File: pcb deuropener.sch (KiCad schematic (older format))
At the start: 30 parts, among them J1 Conn_01x02, J10 Conn_01x03, J11 Barrel_Jack_Switch, J12 Conn_01x08, J13 Conn_01x02, J14 Conn_01x02, J2 Conn_01x02, J3 Conn_01x02, J4 Conn_01x02, J8 Conn_01x02, P8 BeagleBone_Black_Header, P9 BeagleBone_Black_Header, Q1 STU60N3LH5, U1 TSR_1-2450

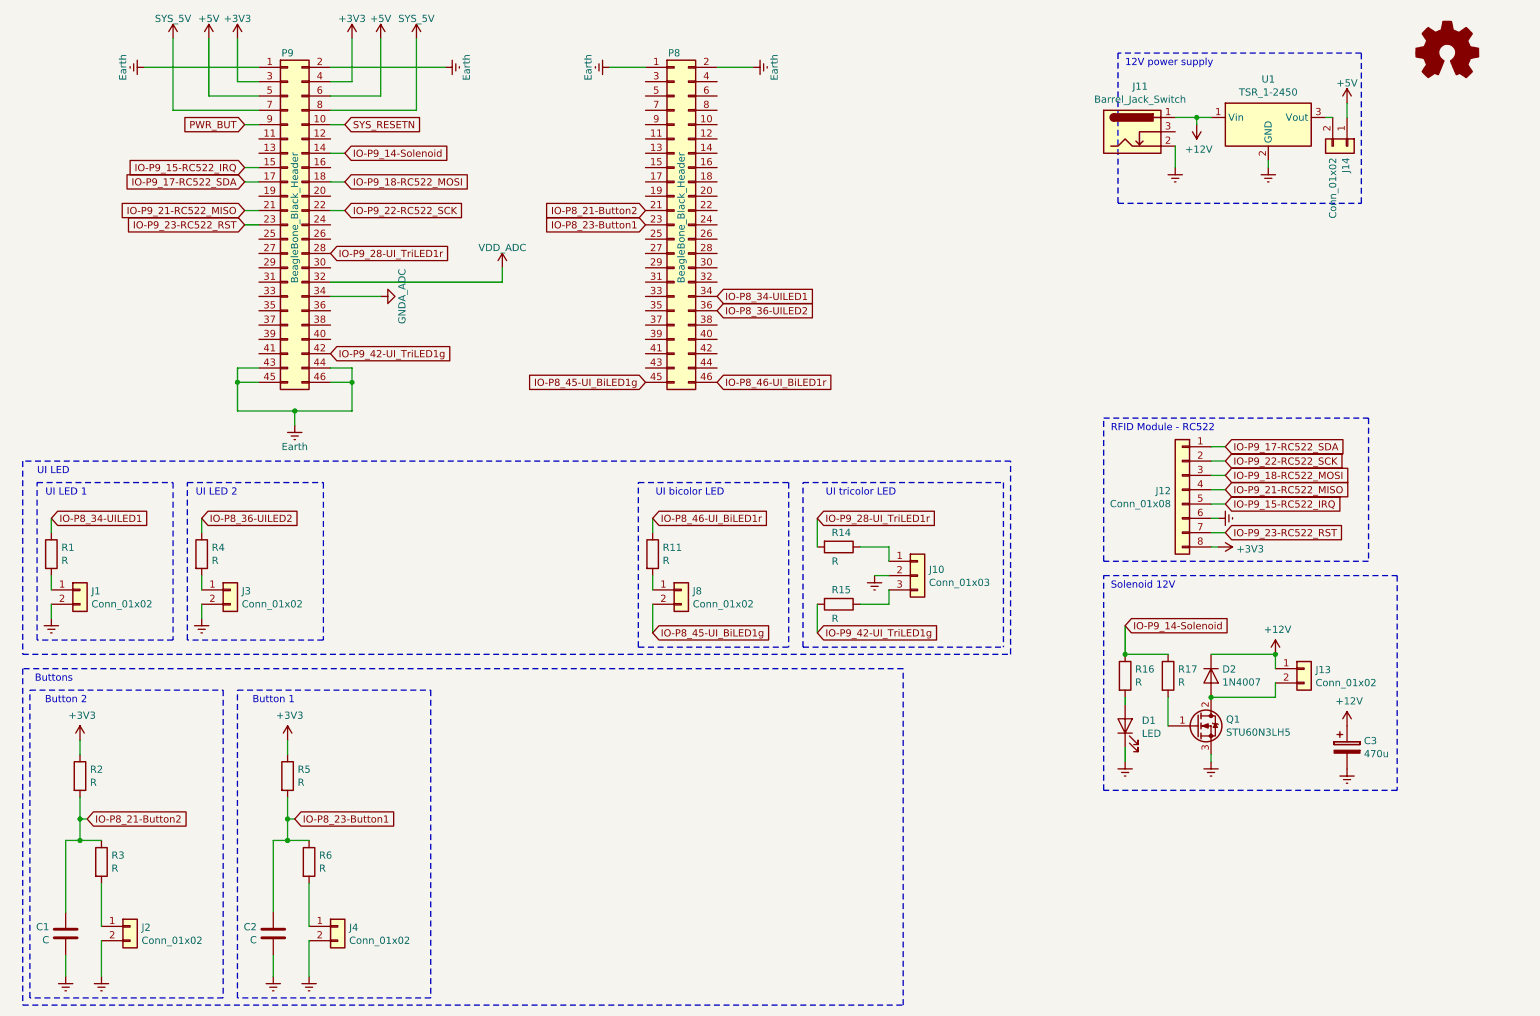
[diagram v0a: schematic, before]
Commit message: A lot of changes to rev 0.02
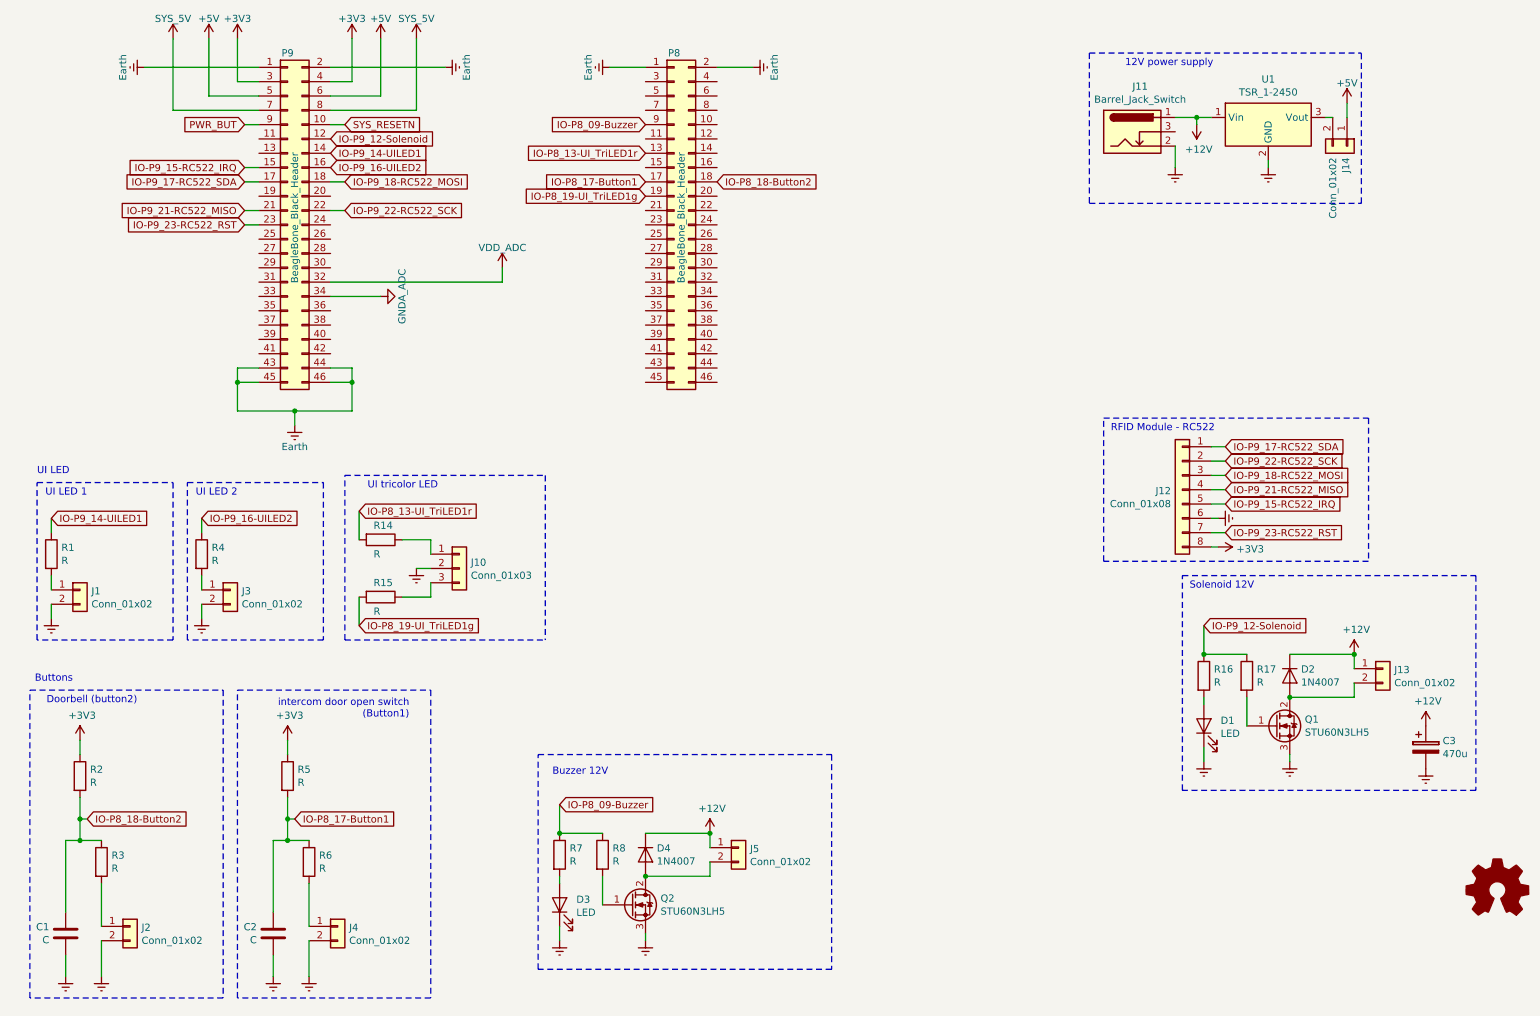
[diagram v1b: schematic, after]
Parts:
- removed J8: Conn_01x02, Connector_PinHeader_2.54mm:PinHeader_1x02_P2.54mm_Vertical, symbol Connector_Generic:Conn_01x02
- removed R11: R, Resistor_THT:R_Axial_DIN0207_L6.3mm_D2.5mm_P10.16mm_Horizontal, symbol Device:R
- added D3: LED, LED_THT:LED_D5.0mm, symbol Device:LED
- added D4: 1N4007, Diode_THT:D_DO-41_SOD81_P10.16mm_Horizontal, symbol Diode:1N4007
- added J5: Conn_01x02, Connector_PinHeader_2.54mm:PinHeader_1x02_P2.54mm_Vertical, symbol Connector_Generic:Conn_01x02
- added Q2: STU60N3LH5, Package_TO_SOT_THT:SIPAK_Vertical, symbol Device:Q_NMOS_GDS
- added R7, R8: R, Resistor_THT:R_Axial_DIN0207_L6.3mm_D2.5mm_P10.16mm_Horizontal, symbol Device:R
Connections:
- net +12V: now also D4.1 (K), J5.1 (Pin_1)
- net Earth: now also D3.1 (K), Q2.3 (S)
- net IO-P9_12-Solenoid: now reaches P9.12 (Pin_12)
- net IO-P9_12-Solenoid: now also R16.1, R17.1
- net IO-P9_16-UILED2: now reaches P9.16 (Pin_16)
- net IO-P9_16-UILED2: now also R4.1
- net IO-P8_13-UI_TriLED1r: now reaches P8.13 (Pin_13)
- net IO-P8_13-UI_TriLED1r: now also R14.2
- net IO-P8_17-Button1: now reaches P8.17 (Pin_17)
- net IO-P8_17-Button1: now also C2.2, R5.2, R6.1
- net IO-P8_18-Button2: now reaches P8.18 (Pin_18)
- net IO-P8_18-Button2: now also C1.2, R2.2, R3.1
- net IO-P8_19-UI_TriLED1g: now reaches P8.19 (Pin_19)
- net IO-P8_19-UI_TriLED1g: now also R15.2
- net IO-P8_09-Buzzer: now reaches P8.9 (Pin_9)
- net IO-P8_09-Buzzer: now also R7.1, R8.1
- removed net IO-P8_21-Button2: C1.2, P8.21 (Pin_21), R2.2, R3.1
- removed net IO-P8_23-Button1: C2.2, P8.23 (Pin_23), R5.2, R6.1
- net IO-P8_34-UILED1: no longer names the net of P8.34 (Pin_34)
- net IO-P8_34-UILED1: no longer R1.1
- net IO-P8_36-UILED2: no longer names the net of P8.36 (Pin_36)
- net IO-P8_36-UILED2: no longer R4.1
- net IO-P8_45-UI_BiLED1g: no longer names the net of P8.45 (Pin_45)
- net IO-P8_46-UI_BiLED1r: no longer names the net of P8.46 (Pin_46)
- removed net IO-P9_14-Solenoid: P9.14 (Pin_14), R16.1, R17.1
- net IO-P9_28-UI_TriLED1r: no longer names the net of P9.28 (Pin_28)
- net IO-P9_28-UI_TriLED1r: no longer R14.2
- net IO-P9_42-UI_TriLED1g: no longer names the net of P9.42 (Pin_42)
- net IO-P9_42-UI_TriLED1g: no longer R15.2
- new net: D3.2 (A), R7.2
- new net: Q2.1 (G), R8.2
- new net: D4.2 (A), J5.2 (Pin_2), Q2.2 (D)
- new net IO-P9_14-UILED1: P9.14 (Pin_14), R1.1
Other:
- note added: "Buzzer 12V"
- note added: "Doorbell (button2)"
- note added: "intercom door open switch \n(Button1)"
- note removed: "Button 1"
- note removed: "Button 2"
- note removed: "UI bicolor LED"
- moved on the sheet: C3, D1, D2, J10, J13, Q1, R14, R15, R16, R17
